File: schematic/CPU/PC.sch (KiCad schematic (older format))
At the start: 70 parts, among them U52 74LS86, U53 74LS08, U54 74LS86, U55 74LS08, U56 74LS273, U57 74LS157, U58 74LS157, U59 74LS32, U60 74LS245

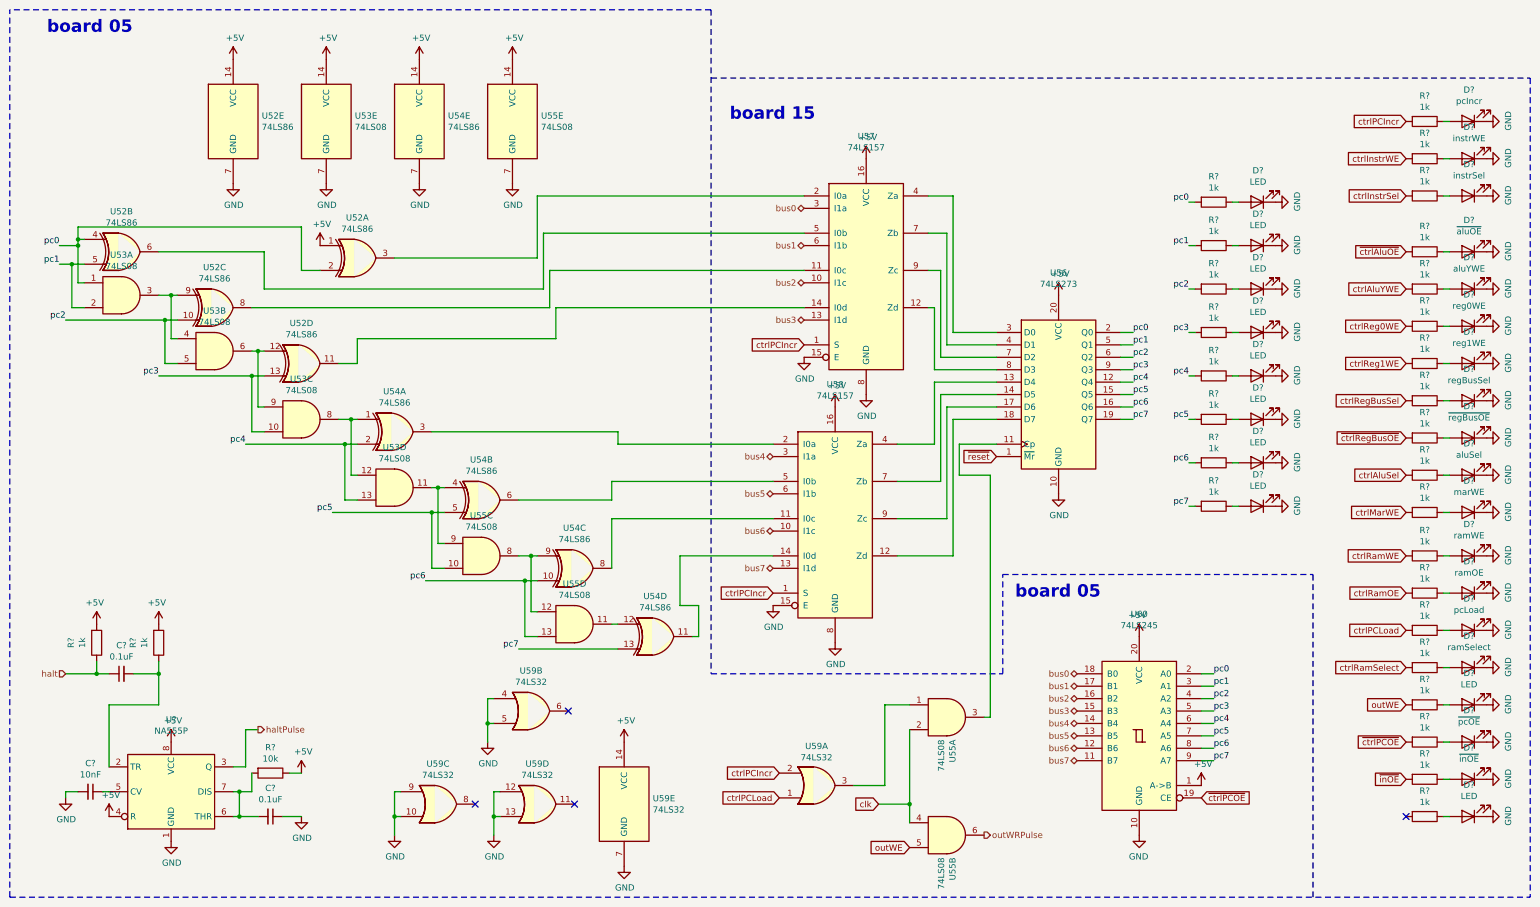
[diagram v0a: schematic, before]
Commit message: pre upgrade to vivado 2021
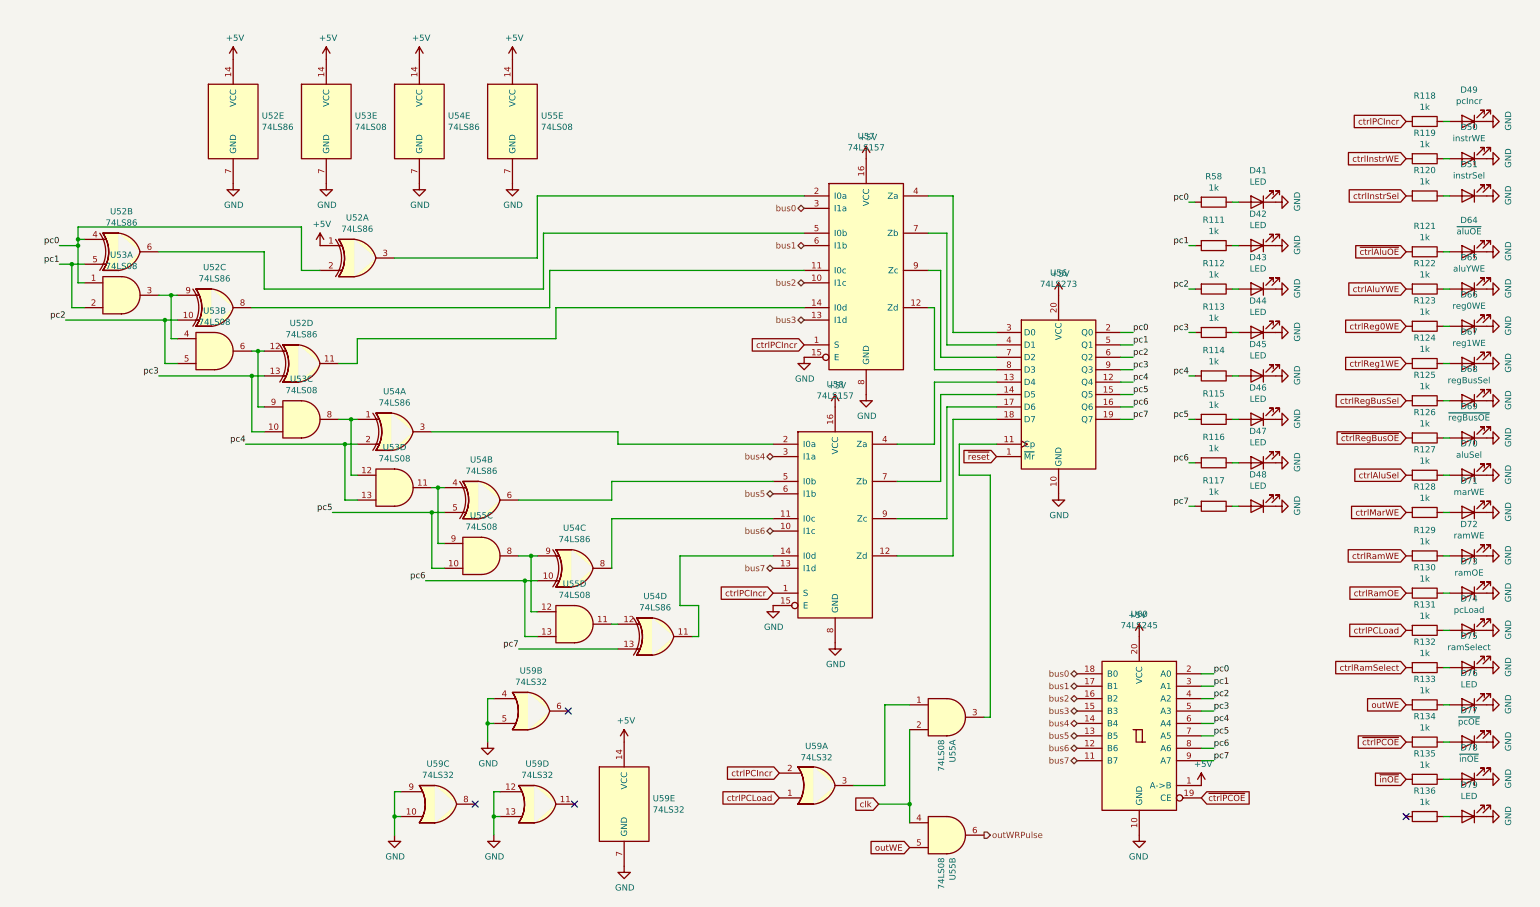
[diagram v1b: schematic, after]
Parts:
- removed C? (x2): 0.1uF, symbol Device:C_Small
- removed C?: 10nF, symbol Device:C_Small
- removed R? (x2): 1k, Resistor_THT:R_Axial_DIN0207_L6.3mm_D2.5mm_P7.62mm_Horizontal, symbol Device:R
- removed R?: 10k, Resistor_THT:R_Axial_DIN0207_L6.3mm_D2.5mm_P7.62mm_Horizontal, symbol Device:R
- removed U?: NA555P, Package_DIP:DIP-8_W7.62mm, symbol Timer:NA555P
- gave numbers to parts that had none: 54
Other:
- note removed: "board 05"
- note removed: "board 15"
